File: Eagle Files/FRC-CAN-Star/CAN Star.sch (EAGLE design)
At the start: 12 parts

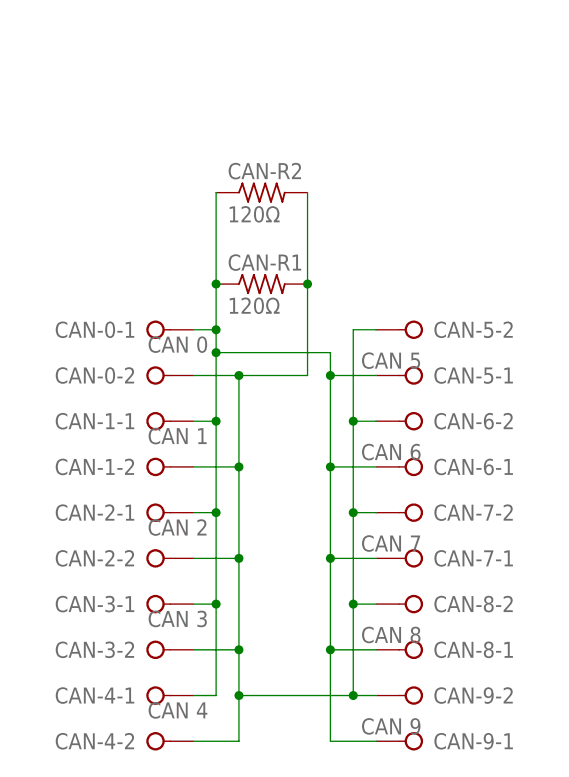
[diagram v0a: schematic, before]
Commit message: Updated Eagle Files
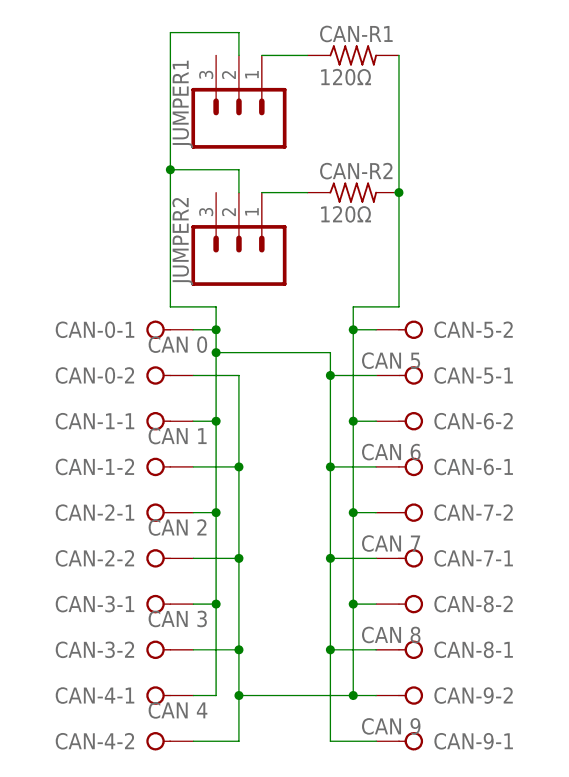
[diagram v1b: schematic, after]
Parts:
- added JUMPER1, JUMPER2: (no value), SparkFun-Connectors:CONN_03
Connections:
- new net N$1: CAN-R1.1, JUMPER1.1
- new net N$2: CAN-R2.1, JUMPER2.1
- net CAN-A: now also JUMPER1.2, JUMPER2.2; no longer CAN-R1.1, CAN-R2.1
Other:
- moved on the sheet: CAN-R1, CAN-R2
